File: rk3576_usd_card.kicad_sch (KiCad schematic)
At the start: 2 parts, among them U27 RK3576

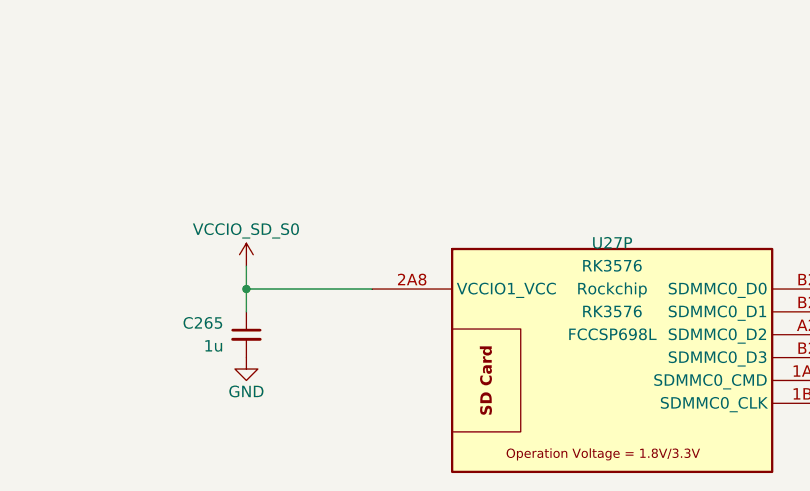
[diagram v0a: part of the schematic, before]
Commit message: Add files via upload
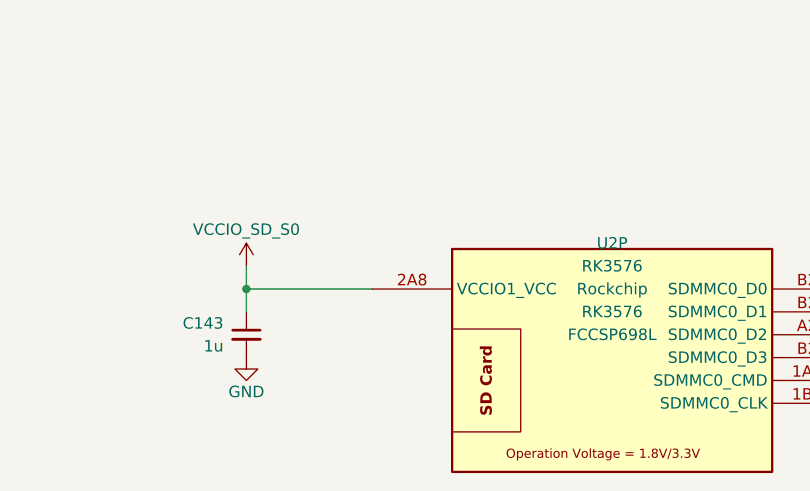
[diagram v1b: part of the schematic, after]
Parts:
- renumbered C265 to C143, U27 to U2
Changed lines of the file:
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@@
 		(dnp no)
 		(fields_autoplaced yes)
-		(property "Reference" "C265"
+		(property "Reference" "C143"
 			(at 58.42 71.1262 0)
 			(show_name no)
@@
 		)
 		(property "Description" "Unpolarized capacitor, small symbol"
+			(at 60.96 72.39 0)
+			(hide yes)
+			(show_name no)
+			(do_not_autoplace no)
+			(effects
+				(font
+					(size 1.27 1.27)
+				)
+			)
+		)
+		(property "Dielectric" ""
+			(at 60.96 72.39 0)
+			(hide yes)
+			(show_name no)
+			(do_not_autoplace no)
+			(effects
+				(font
+					(size 1.27 1.27)
+				)
+			)
+		)
+		(property "Voltage" ""
+			(at 60.96 72.39 0)
+			(hide yes)
+			(show_name no)
+			(do_not_autoplace no)
+			(effects
+				(font
+					(size 1.27 1.27)
+				)
+			)
+		)
+		(property "KLC_S3.3" ""
+			(at 60.96 72.39 0)
+			(hide yes)
+			(show_name no)
+			(do_not_autoplace no)
+			(effects
+				(font
+					(size 1.27 1.27)
+				)
+			)
+		)
+		(property "KLC_S4.1" ""
+			(at 60.96 72.39 0)
+			(hide yes)
+			(show_name no)
+			(do_not_autoplace no)
+			(effects
+				(font
+					(size 1.27 1.27)
+				)
+			)
+		)
+		(property "KLC_S5.1" ""
 			(at 60.96 72.39 0)
 			(hide yes)
@@
 			(project "RK3576 SBC"
 				(path "/b79dbff4-0cad-4ff7-bec2-7c0e4f8b14d3/34f9b0cb-aeae-42b4-a2af-a0a79afcf392/e3169b31-7633-42aa-8b59-c93f8fc73ecf"
-					(reference "C265")
+					(reference "C143")
 					(unit 1)
 				)
@@
 		(in_pos_files yes)
 		(dnp no)
-		(property "Reference" "#PWR0352"
+		(property "Reference" "#PWR0205"
 			(at 60.96 81.28 0)
 			(hide yes)
@@
 			(project "RK3576 SBC"
 				(path "/b79dbff4-0cad-4ff7-bec2-7c0e4f8b14d3/34f9b0cb-aeae-42b4-a2af-a0a79afcf392/e3169b31-7633-42aa-8b59-c93f8fc73ecf"
-					(reference "#PWR0352")
+					(reference "#PWR0205")
 					(unit 1)
 				)
@@
 		(in_pos_files yes)
 		(dnp no)
-		(property "Reference" "#PWR0351"
+		(property "Reference" "#PWR0204"
 			(at 60.96 68.58 0)
 			(hide yes)
@@
 			(project "RK3576 SBC"
 				(path "/b79dbff4-0cad-4ff7-bec2-7c0e4f8b14d3/34f9b0cb-aeae-42b4-a2af-a0a79afcf392/e3169b31-7633-42aa-8b59-c93f8fc73ecf"
-					(reference "#PWR0351")
+					(reference "#PWR0204")
 					(unit 1)
 				)
@@
 		(dnp no)
 		(fields_autoplaced yes)
-		(property "Reference" "U27"
+		(property "Reference" "U2"
 			(at 101.6 62.23 0)
 			(show_name no)
@@
 		(property "Package" "FCCSP698L"
 			(at 101.6 72.39 0)
+			(show_name no)
+			(do_not_autoplace no)
+			(effects
+				(font
+					(size 1.27 1.27)
+				)
+			)
+		)
+		(property "Dielectric" ""
+			(at 101.6 87.63 0)
+			(hide yes)
+			(show_name no)
+			(do_not_autoplace no)
+			(effects
+				(font
+					(size 1.27 1.27)
+				)
+			)
+		)
+		(property "Voltage" ""
+			(at 101.6 87.63 0)
+			(hide yes)
+			(show_name no)
+			(do_not_autoplace no)
+			(effects
+				(font
+					(size 1.27 1.27)
+				)
+			)
+		)
+		(property "KLC_S3.3" ""
+			(at 101.6 87.63 0)
+			(hide yes)
+			(show_name no)
+			(do_not_autoplace no)
+			(effects
+				(font
+					(size 1.27 1.27)
+				)
+			)
+		)
+		(property "KLC_S4.1" ""
+			(at 101.6 87.63 0)
+			(hide yes)
+			(show_name no)
+			(do_not_autoplace no)
+			(effects
+				(font
+					(size 1.27 1.27)
+				)
+			)
+		)
+		(property "KLC_S5.1" ""
+			(at 101.6 87.63 0)
+			(hide yes)
 			(show_name no)
 			(do_not_autoplace no)
@@
 			(project "RK3576 SBC"
 				(path "/b79dbff4-0cad-4ff7-bec2-7c0e4f8b14d3/34f9b0cb-aeae-42b4-a2af-a0a79afcf392/e3169b31-7633-42aa-8b59-c93f8fc73ecf"
-					(reference "U27")
+					(reference "U2")
 					(unit 16)
 				)
